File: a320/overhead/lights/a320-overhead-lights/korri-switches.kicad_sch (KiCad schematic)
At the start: 30 parts

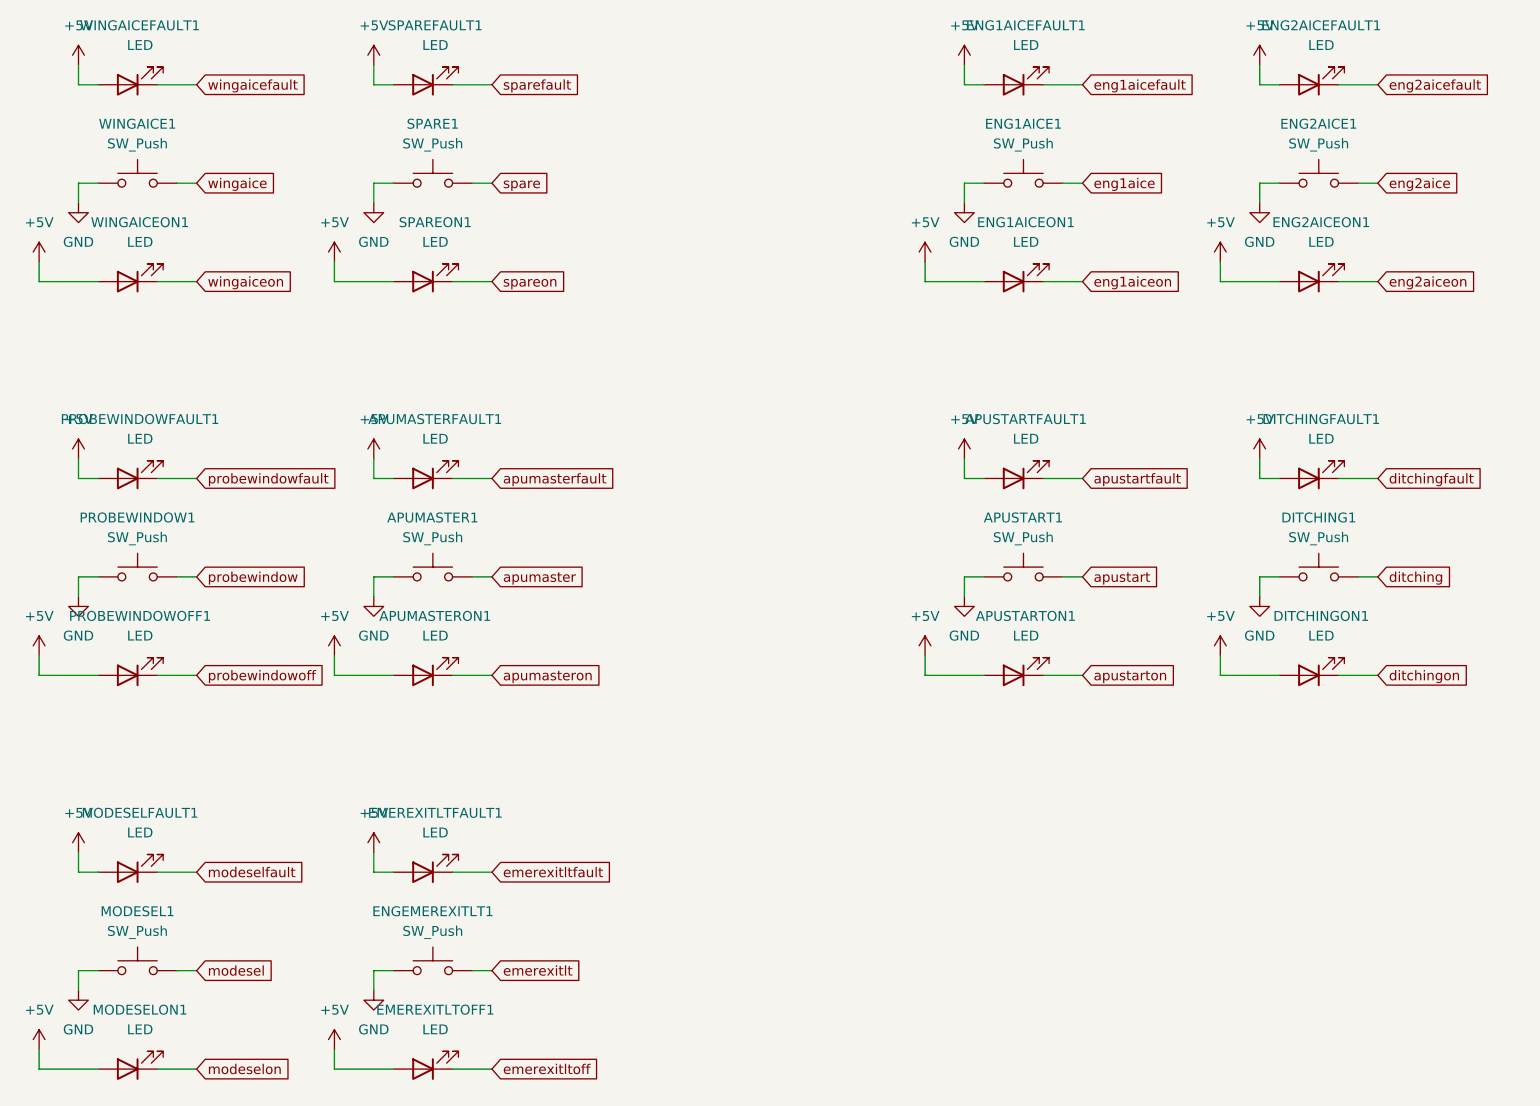
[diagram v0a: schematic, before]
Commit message: misc
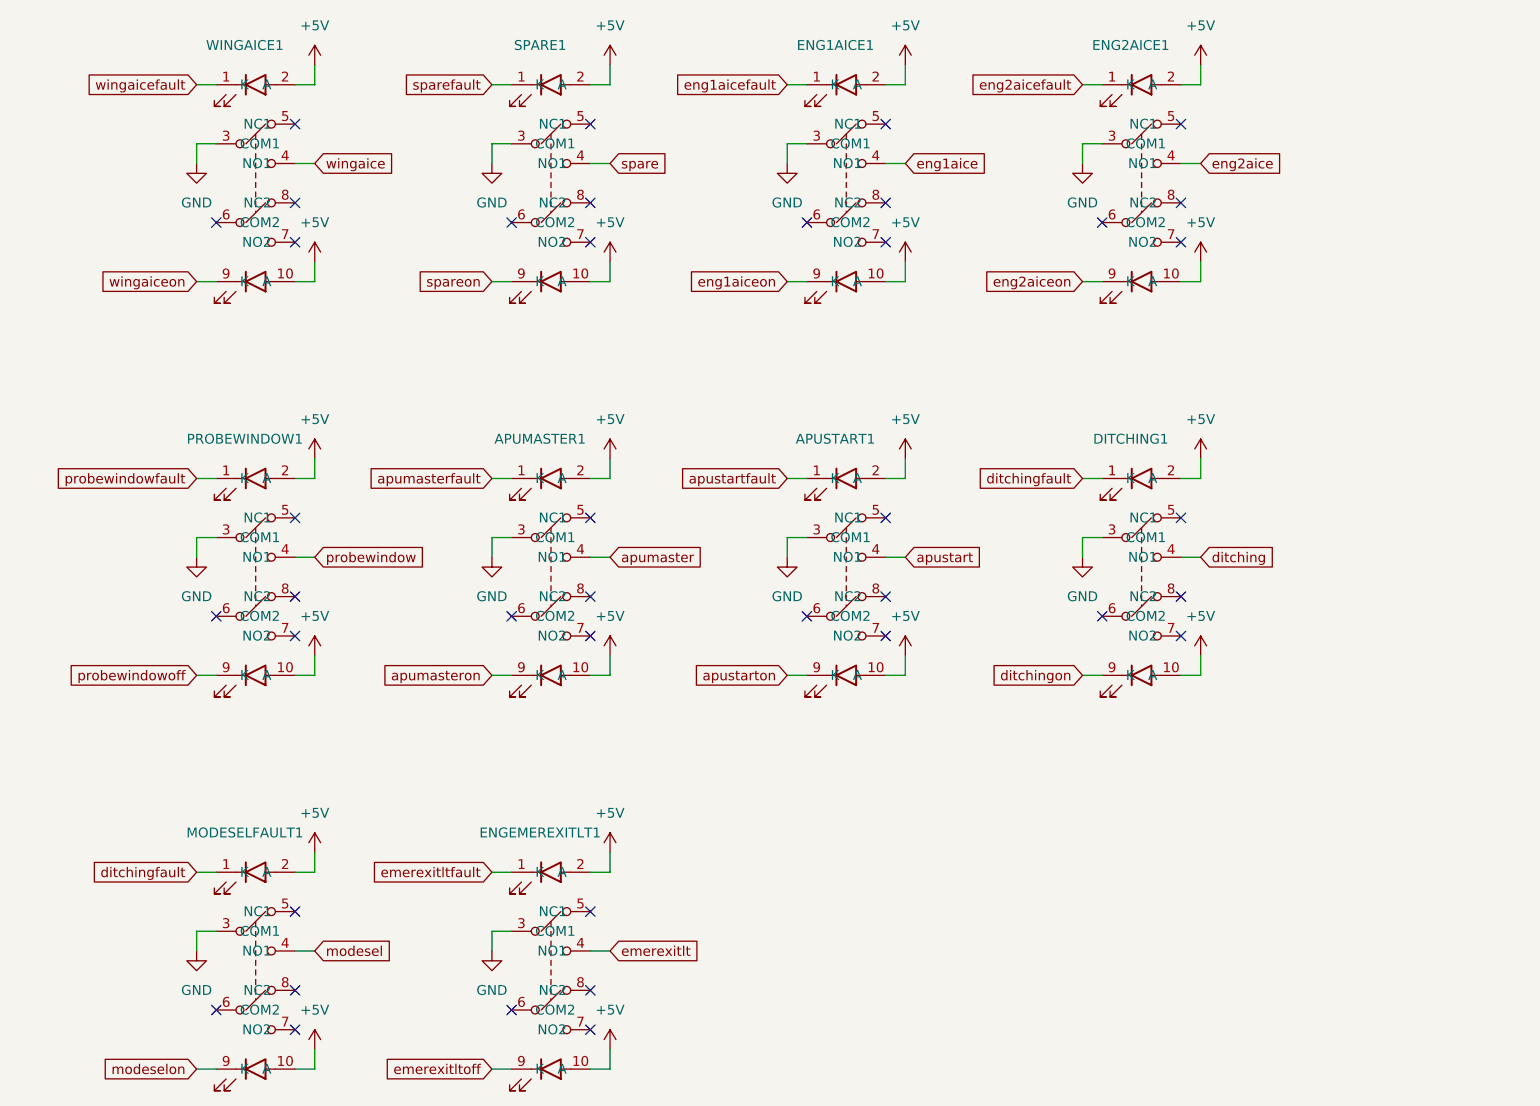
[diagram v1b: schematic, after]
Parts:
- removed APUMASTER1, APUSTART1, DITCHING1, ENG1AICE1, ENG2AICE1, ENGEMEREXITLT1, MODESEL1, PROBEWINDOW1, SPARE1, WINGAICE1: SW_Push, symbol Switch:SW_Push
- removed APUMASTERFAULT1, APUMASTERON1, APUSTARTFAULT1, APUSTARTON1, DITCHINGFAULT1, DITCHINGON1, EMEREXITLTFAULT1, EMEREXITLTOFF1, ENG1AICEFAULT1, ENG1AICEON1, ENG2AICEFAULT1, ENG2AICEON1, MODESELFAULT1, MODESELON1, PROBEWINDOWFAULT1, PROBEWINDOWOFF1, SPAREFAULT1, SPAREON1, WINGAICEFAULT1, WINGAICEON1: LED, symbol Device:LED
- added APUMASTER1, APUSTART1, DITCHING1, ENG1AICE1, ENG2AICE1, ENGEMEREXITLT1, MODESELFAULT1, PROBEWINDOW1, SPARE1, WINGAICE1: ~, a320:Korry Switch, symbol a320:Korry_Switch
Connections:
- net +5V: now also APUMASTER1.10 (A), APUMASTER1.2 (A), APUSTART1.10 (A), APUSTART1.2 (A), DITCHING1.10 (A), DITCHING1.2 (A), ENG1AICE1.10 (A), ENG1AICE1.2 (A), ENG2AICE1.10 (A), ENG2AICE1.2 (A), ENGEMEREXITLT1.10 (A), ENGEMEREXITLT1.2 (A), MODESELFAULT1.10 (A), MODESELFAULT1.2 (A), PROBEWINDOW1.10 (A), PROBEWINDOW1.2 (A), SPARE1.10 (A), SPARE1.2 (A), WINGAICE1.10 (A), WINGAICE1.2 (A)
- net GND: now also APUMASTER1.3 (COM1), APUSTART1.3 (COM1), DITCHING1.3 (COM1), ENG1AICE1.3 (COM1), ENG2AICE1.3 (COM1), ENGEMEREXITLT1.3 (COM1), MODESELFAULT1.3 (COM1), PROBEWINDOW1.3 (COM1), SPARE1.3 (COM1), WINGAICE1.3 (COM1)
- net apumaster: now also APUMASTER1.4 (NO1)
- net apumasterfault: now also APUMASTER1.1 (K)
- net apumasteron: now also APUMASTER1.9 (K)
- net apustart: now also APUSTART1.4 (NO1)
- net apustartfault: now also APUSTART1.1 (K)
- net apustarton: now also APUSTART1.9 (K)
- net ditching: now also DITCHING1.4 (NO1)
- net ditchingfault: now also DITCHING1.1 (K), MODESELFAULT1.1 (K)
- net ditchingon: now also DITCHING1.9 (K)
- net emerexitlt: now also ENGEMEREXITLT1.4 (NO1)
- net emerexitltfault: now also ENGEMEREXITLT1.1 (K)
- net emerexitltoff: now also ENGEMEREXITLT1.9 (K)
- net eng1aice: now also ENG1AICE1.4 (NO1)
- net eng1aicefault: now also ENG1AICE1.1 (K)
- net eng1aiceon: now also ENG1AICE1.9 (K)
- net eng2aice: now also ENG2AICE1.4 (NO1)
- net eng2aicefault: now also ENG2AICE1.1 (K)
- net eng2aiceon: now also ENG2AICE1.9 (K)
- net modesel: now also MODESELFAULT1.4 (NO1)
- net modeselon: now also MODESELFAULT1.9 (K)
- net probewindow: now also PROBEWINDOW1.4 (NO1)
- net probewindowfault: now also PROBEWINDOW1.1 (K)
- net probewindowoff: now also PROBEWINDOW1.9 (K)
- net spare: now also SPARE1.4 (NO1)
- net sparefault: now also SPARE1.1 (K)
- net spareon: now also SPARE1.9 (K)
- net wingaice: now also WINGAICE1.4 (NO1)
- net wingaicefault: now also WINGAICE1.1 (K)
- net wingaiceon: now also WINGAICE1.9 (K)
- no-connect marks 0 -> 40
